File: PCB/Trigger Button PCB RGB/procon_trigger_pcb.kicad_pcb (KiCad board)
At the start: 2 copper layers, 110.3 x 46.3 mm, 10 parts, among them J1 Conn_01x05_Pin, J2 Conn_01x05_Pin, SW1 SW_Push, SW2 SW_Push, SW3 SW_Push, SW4 SW_Push

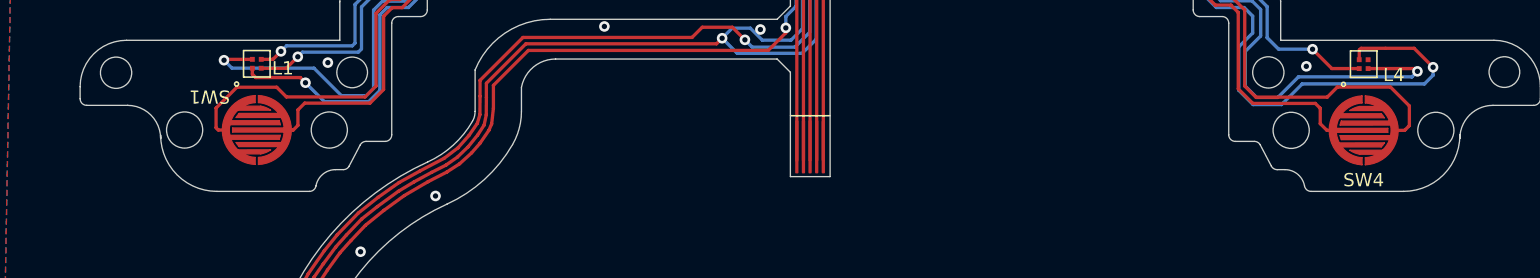
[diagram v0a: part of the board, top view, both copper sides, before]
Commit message: Update component BOM and production files.
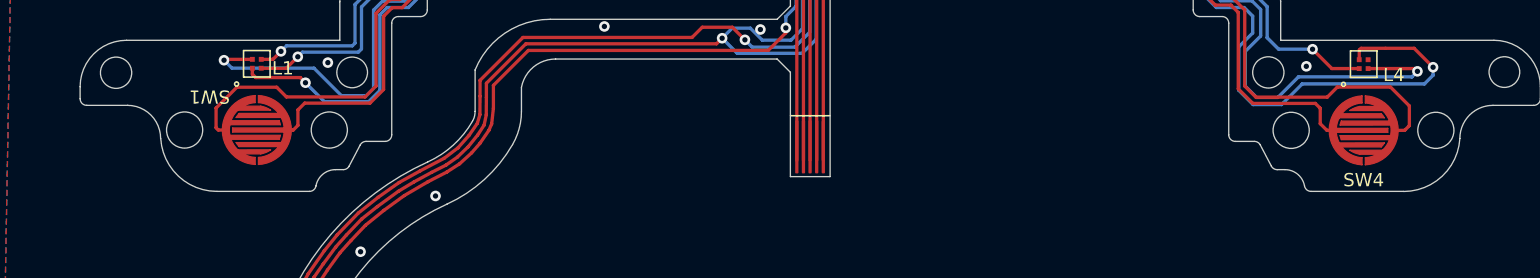
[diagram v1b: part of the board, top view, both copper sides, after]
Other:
- outline, holes or cut-outs redrawn
